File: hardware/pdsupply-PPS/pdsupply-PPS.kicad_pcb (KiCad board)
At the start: 4 copper layers, 44 x 36.5 mm, 74 parts, among them IC1 LTM8083EY#PBF, IC2 FPF2895UCX, J1 USB4505-03-0-A_REVA, J2 USB4505-03-0-A_REVA, J3 Screw_Terminal_01x02, U1 FUSB307BMPX, U2 ADUM3160, U3 ACS71240KEXBLT-050U5, U4 STM32L432KCUx

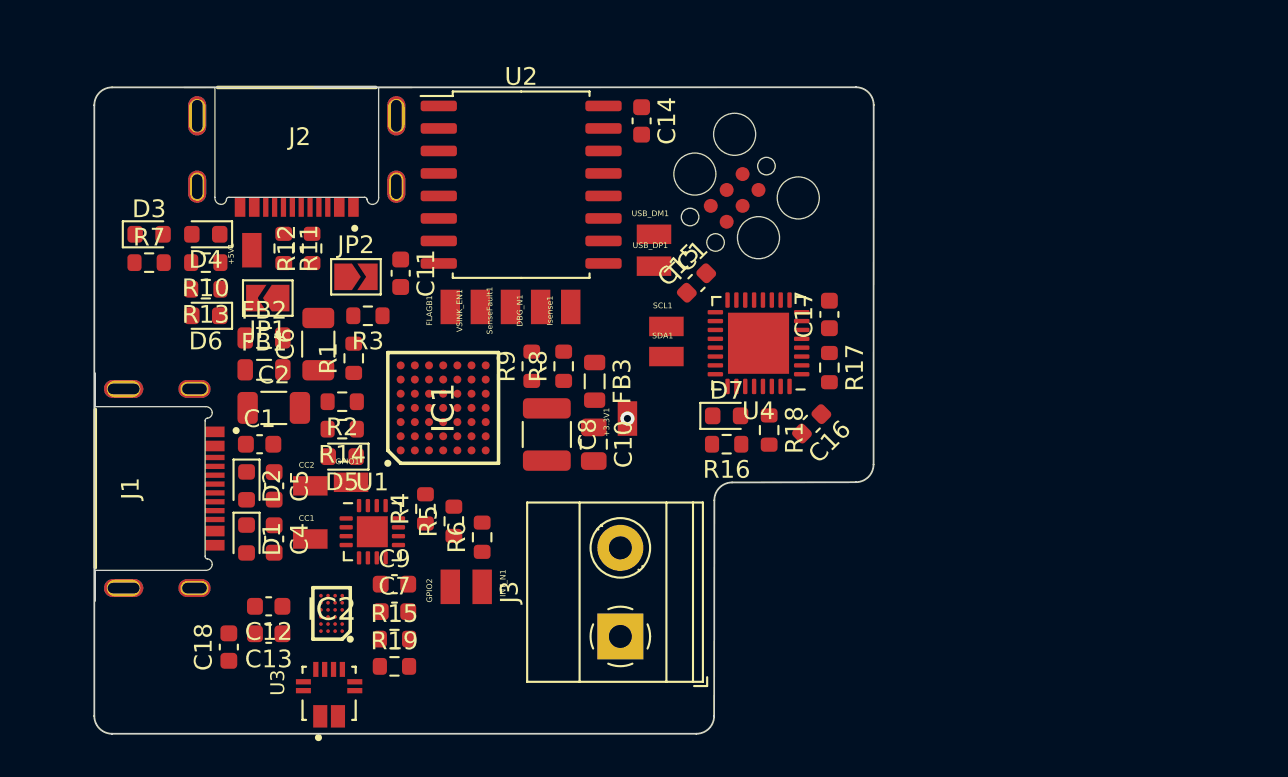
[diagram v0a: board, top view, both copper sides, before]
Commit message: added few routes
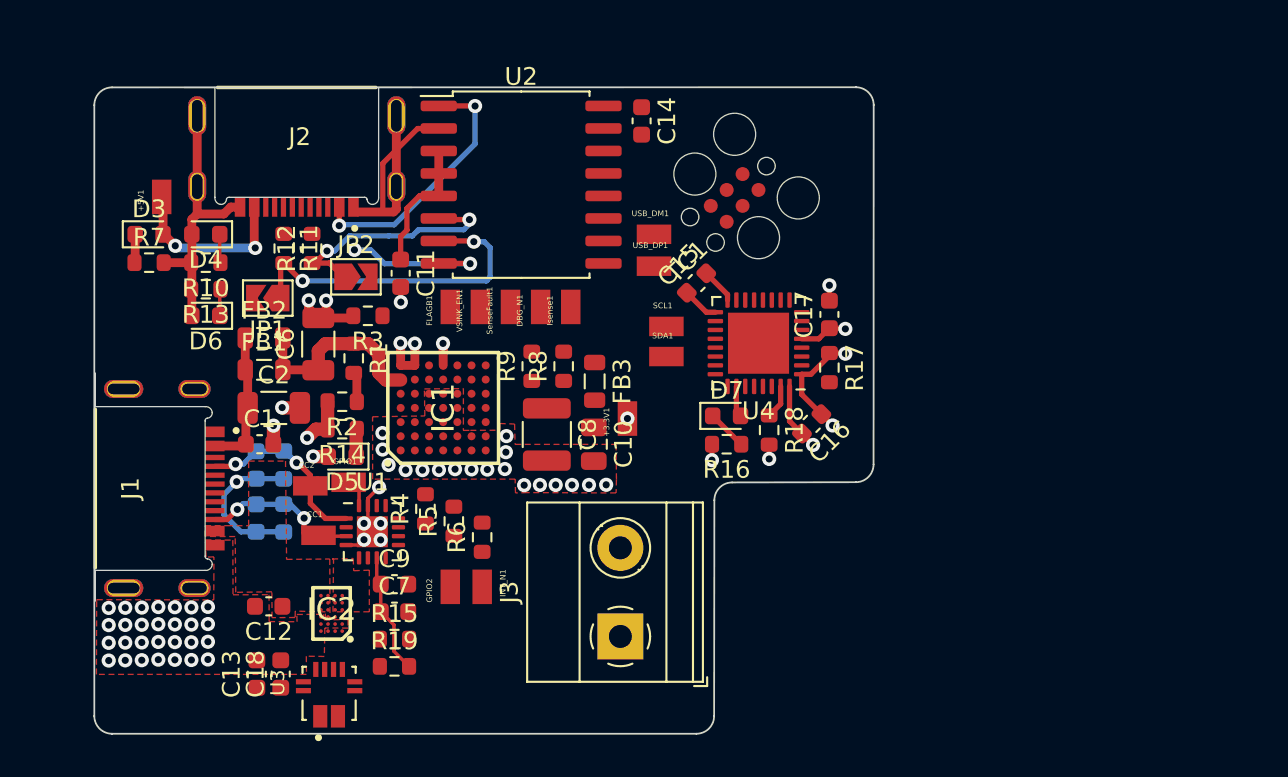
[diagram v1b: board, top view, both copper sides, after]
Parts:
- C4, C5, D1, D2: moved to B.Cu
- moved +5V1 5.91 mm to (113.8, 89.7)
- moved C18 3.30 mm to (120.5, 116.6)
- moved D1 2.41 mm to (120.7, 107.8)
- moved D2 2.41 mm to (120.7, 104.8)
- moved C13 2.37 mm to (119.2, 116.6), turned to 90 degrees
- moved C4 1.56 mm to (119.1, 107.8)
- moved C5 1.56 mm to (119.1, 104.8)
- moved CC1 0.51 mm to (122.7, 108.8)
- moved GPIO1 0.14 mm to (124.4, 105.8)
- turned R1 to -90 degrees
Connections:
- net Net-(C13-Pad1) renamed /Vbus_pre
- net Net-(J3-Pad1) renamed /VBus_Out
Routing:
- net GND1: track 0.00 -> 39.5 mm, vias 0 -> 3
- net GND: track 0.00 -> 35.1 mm, vias 0 -> 64
- net +5V: track 0.00 -> 24.9 mm, vias 0 -> 4
- net +3V3: track 0.00 -> 19.6 mm, vias 1 -> 5
- net Net-(JP1-Pad1): track 0.00 -> 18.9 mm, vias 0 -> 2
- net Net-(JP2-Pad1): track 0.00 -> 13.9 mm, vias 0 -> 2
- net Net-(C6-Pad1): track 0.00 -> 11.2 mm
- net /CC1: track 0.00 -> 10.7 mm, vias 0 -> 2
- net /CC2: track 0.00 -> 9.19 mm, vias 0 -> 2
- net VBUS: track 0.00 -> 8.20 mm
- net Net-(C11-Pad1): track 0.00 -> 7.66 mm
- net Net-(D7-Pad1): track 0.00 -> 2.28 mm
- net Net-(IC1-PadB6): track 0.00 -> 1.91 mm
- net Net-(R18-Pad1): track 0.00 -> 1.91 mm
- net Net-(D7-Pad2): track 0.00 -> 1.76 mm
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- added copper zone on F.Cu, net /Vbus_pre
- added copper zone on F.Cu, net GND
- added copper zone on F.Cu, net VBUS

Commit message: almost done with routing
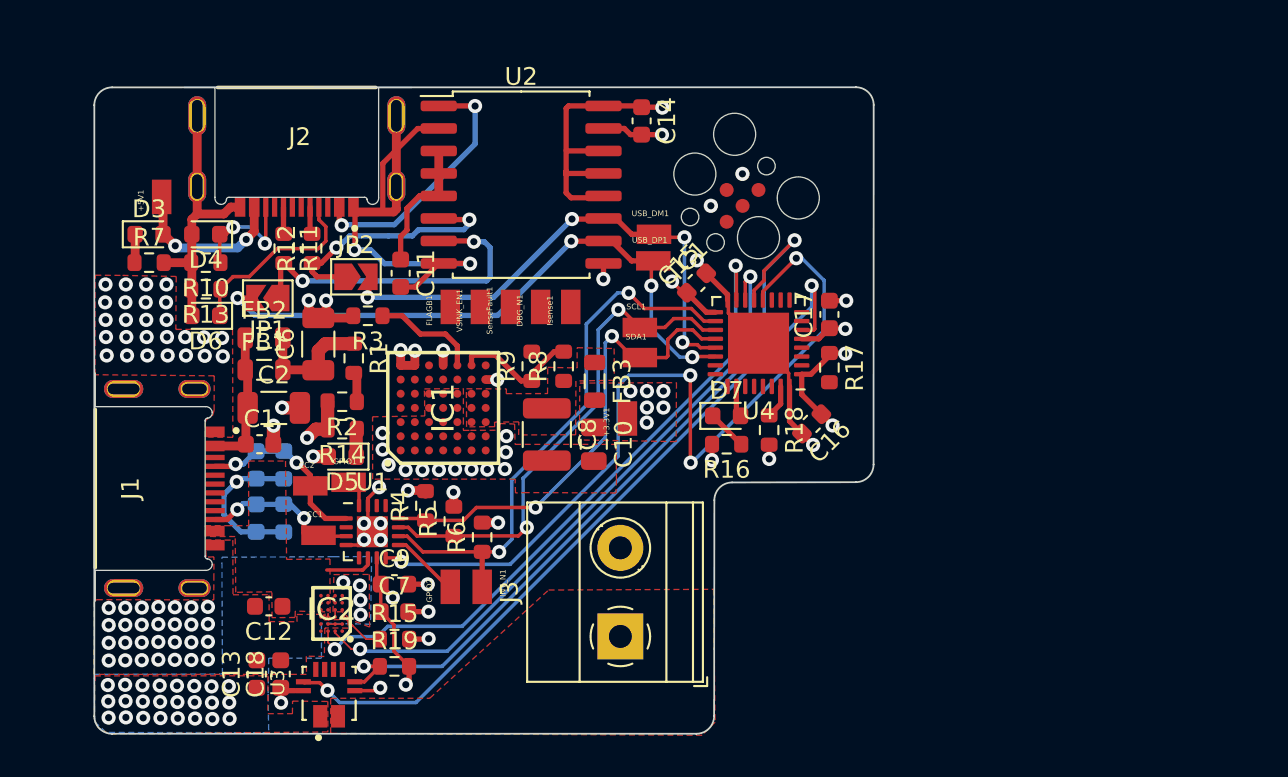
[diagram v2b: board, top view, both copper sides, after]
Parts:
- moved SCL1 1.50 mm to (140.8, 97.1)
- moved SDA1 1.50 mm to (140.8, 98.8)
- moved USB_DP1 0.30 mm to (141.6, 93.3)
- moved R4 0.17 mm to (128.7, 107.1)
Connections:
- net Net-(C8-Pad1) renamed /+3.3V_Pre
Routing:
- net /DBG_N: track 0.00 -> 47.7 mm, vias 0 -> 4
- net /SenseFault: track 0.00 -> 43.7 mm, vias 0 -> 2
- net /Isense: track 0.00 -> 42.8 mm, vias 0 -> 2
- net /FLAGB: track 0.00 -> 37.6 mm, vias 0 -> 2
- net /VSINK_EN: track 0.00 -> 36.5 mm, vias 0 -> 2
- net /USB_DP: track 0.00 -> 35.2 mm, vias 0 -> 4
- net /INT_N: track 0.00 -> 31.6 mm, vias 0 -> 2
- net /USB_DM: track 0.00 -> 29.8 mm, vias 0 -> 4
- net /SCL: track 0.00 -> 28.6 mm, vias 0 -> 2
- net /SDA: track 0.00 -> 27.0 mm, vias 0 -> 2
- net +3V3: track 19.6 -> 44.4 mm, vias 5 -> 19
- net GND: track 35.1 -> 53.4 mm, vias 64 -> 93
- net Net-(D6-Pad1): track 1.52 -> 10.7 mm
- net Net-(IC1-PadF7): track 0.00 -> 7.25 mm
- net Net-(IC1-PadE7): track 0.00 -> 6.03 mm
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- added copper zone on F.Cu, net +3V3
- added copper zone on F.Cu, net /+3.3V_Pre
- added copper zone on F.Cu, net /VBus_Out
- added copper zone on B.Cu, net /Vbus_pre

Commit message: almost done
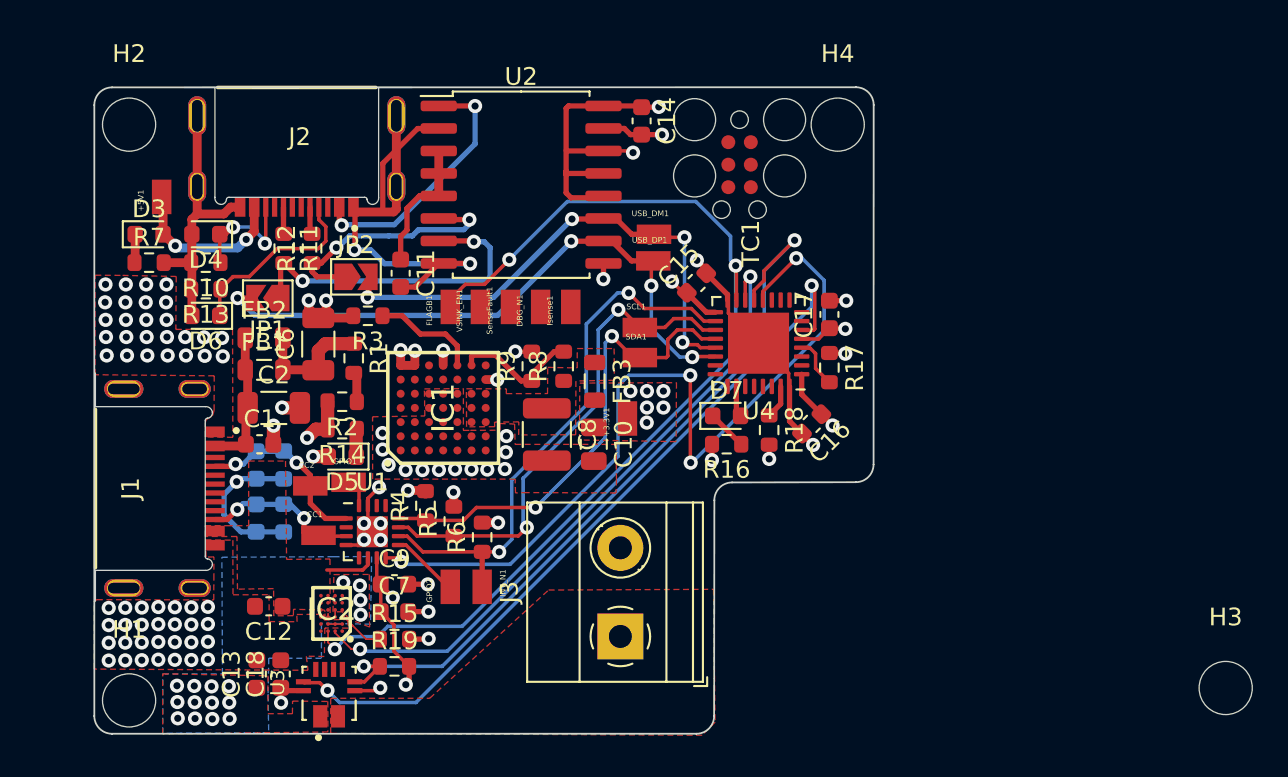
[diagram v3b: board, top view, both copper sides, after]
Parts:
- added H1: MountingHole_Pad, MountingHole:MountingHole_3mm, F.Cu at (112.0, 118.1)
- added H2: MountingHole_Pad, MountingHole:MountingHole_3mm, F.Cu at (112.0, 85.6)
- added H3: MountingHole_Pad, MountingHole:MountingHole_3mm, F.Cu at (173.9, 117.4)
- added H4: MountingHole_Pad, MountingHole:MountingHole_3mm, F.Cu at (152.0, 85.6)
- moved TC1 1.90 mm to (146.4, 87.9), turned to -90 degrees
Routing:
- net /FLAGB: track 37.6 -> 58.7 mm, vias 2 -> 3
- net Net-(R17-Pad2): track 0.00 -> 2.86 mm
- net GND: track 53.4 -> 54.4 mm
- net /Vbus_pre: vias 28 -> 16

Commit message: added holes
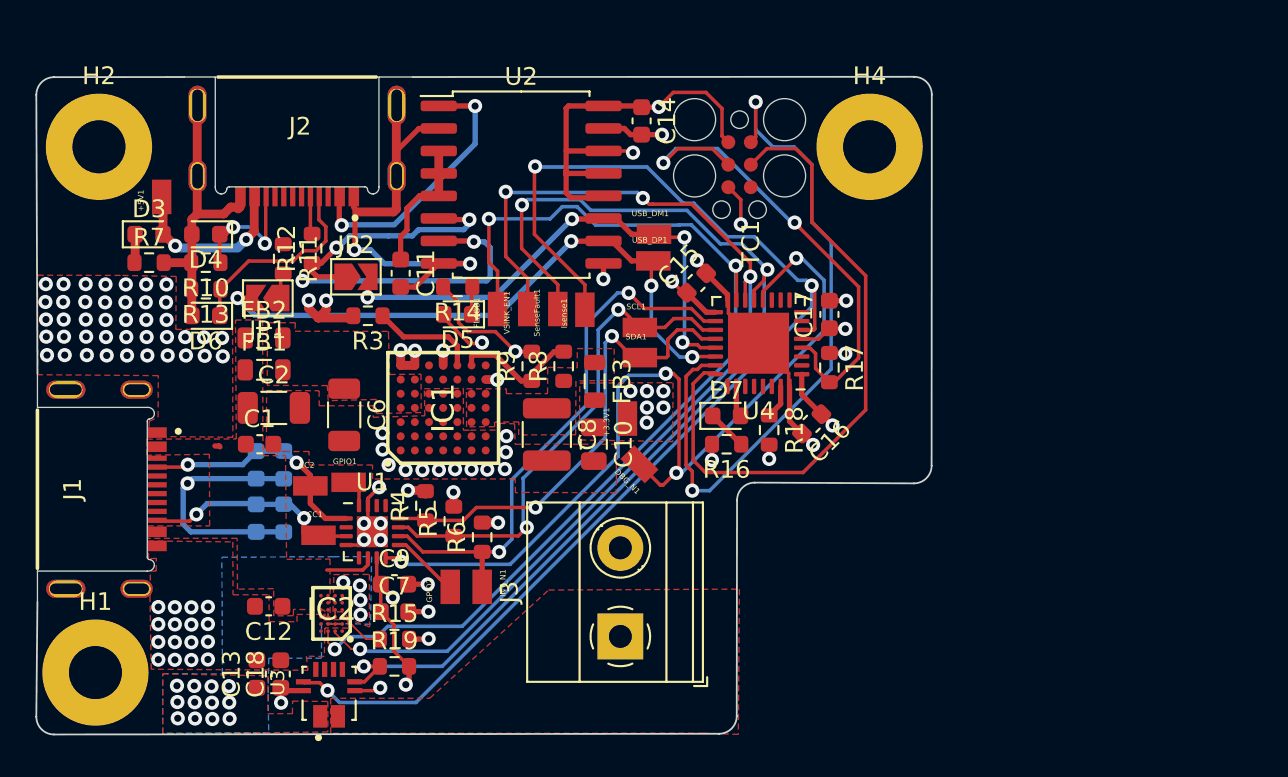
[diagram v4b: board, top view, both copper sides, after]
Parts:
- removed H3: MountingHole_Pad, MountingHole:MountingHole_3mm
- removed R1: 200k, Resistor_SMD:R_0603_1608Metric
- removed R2: 270k, Resistor_SMD:R_0603_1608Metric
- H1, H2, H4: footprint MountingHole:MountingHole_3mm -> MountingHole:MountingHole_3mm_Pad
- moved DBG_N1 10.5 mm to (140.8, 104.8), turned to 135 degrees
- moved D5 10.3 mm to (130.5, 96.3)
- moved R14 10.3 mm to (130.5, 94.8)
- moved C6 4.25 mm to (124.1, 102.0), turned to -90 degrees
- moved J1 3.27 mm to (108.4, 106.2)
- moved FLAGB1 2.67 mm to (132.8, 96.0)
- moved SenseFault1 2.67 mm to (136.2, 96.0)
- moved VSINK_EN1 2.67 mm to (134.5, 96.0)
- moved H1 2.46 mm to (110.1, 116.5)
- moved H4 2.19 mm to (153.8, 86.9)
- moved H2 2.11 mm to (110.3, 86.9)
- moved Isense1 0.82 mm to (137.7, 96.1)
- moved J2 0.59 mm to (121.5, 84.5)
- moved R11 0.59 mm to (120.7, 93.2)
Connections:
- C6 pad 1: Net-(C6-Pad1) -> /VBUS_Rdy
- FB1 pad 2: Net-(C6-Pad1) -> /VBUS_Rdy
- FB2 pad 2: Net-(C6-Pad1) -> /VBUS_Rdy
- IC1 pad A1: GND -> Net-(IC1-PadA1)
- IC1 pad A2: GND -> Net-(IC1-PadA1)
- IC1 pad A3: GND -> Net-(IC1-PadA1)
- IC1 pad A4: Net-(C6-Pad1) -> /VBUS_Rdy
- IC1 pad A5: Net-(C6-Pad1) -> /VBUS_Rdy
- IC1 pad A6: Net-(C6-Pad1) -> /VBUS_Rdy
- IC1 pad A7: GND -> Net-(IC1-PadA1)
- IC1 pad B1: GND -> Net-(IC1-PadA1)
- IC1 pad B2: GND -> Net-(IC1-PadA1)
- IC1 pad B3: GND -> Net-(IC1-PadA1)
- IC1 pad B4: Net-(C6-Pad1) -> /VBUS_Rdy
- IC1 pad B5: Net-(C6-Pad1) -> /VBUS_Rdy
- IC1 pad B6: Net-(IC1-PadB6) -> /VBUS_Rdy
- IC1 pad B7: GND -> Net-(IC1-PadA1)
- IC1 pad C1: GND -> Net-(IC1-PadA1)
- IC1 pad C2: GND -> Net-(IC1-PadA1)
- IC1 pad C3: GND -> Net-(IC1-PadA1)
- IC1 pad C4: GND -> Net-(IC1-PadA1)
- IC1 pad C5: GND -> Net-(IC1-PadA1)
- IC1 pad D1: GND -> Net-(IC1-PadA1)
- IC1 pad D2: GND -> Net-(IC1-PadA1)
- IC1 pad D3: GND -> Net-(IC1-PadA1)
- IC1 pad D4: GND -> Net-(IC1-PadA1)
- IC1 pad D5: GND -> Net-(IC1-PadA1)
- IC1 pad D7: GND -> Net-(IC1-PadA1)
- IC1 pad E1: GND -> Net-(IC1-PadA1)
- IC1 pad E2: GND -> Net-(IC1-PadA1)
- IC1 pad E3: GND -> Net-(IC1-PadA1)
- IC1 pad E4: GND -> Net-(IC1-PadA1)
- IC1 pad E5: GND -> Net-(IC1-PadA1)
- IC1 pad F1: GND -> Net-(IC1-PadA1)
- IC1 pad F2: GND -> Net-(IC1-PadA1)
- IC1 pad G1: GND -> Net-(IC1-PadA1)
- IC1 pad G2: GND -> Net-(IC1-PadA1)
- IC1 pad G6: GND -> Net-(IC1-PadA1)
- R3 pad 2: GND -> Net-(IC1-PadA1)
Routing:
- net Net-(TC1-Pad2): track 0.00 -> 39.1 mm, vias 0 -> 2
- net Net-(TC1-Pad4): track 0.00 -> 36.7 mm
- net /Isense: track 42.8 -> 70.4 mm, vias 2 -> 3
- net Net-(R17-Pad2): track 2.86 -> 28.1 mm, vias 0 -> 2
- net /VSINK_EN: track 36.5 -> 59.9 mm, vias 2 -> 4
- net /SenseFault: track 43.7 -> 61.5 mm, vias 2 -> 3
- net Net-(IC1-PadA1): track 0.00 -> 8.71 mm, vias 0 -> 6
- net +3V3: track 43.9 -> 52.4 mm
- net VBUS: track 11.2 -> 3.80 mm
- net Net-(C6-Pad1): track 7.07 -> 0.00 mm
- net /DBG_N: track 47.7 -> 51.6 mm
- net GND1: track 43.7 -> 39.9 mm
- net /CC2: track 9.19 -> 12.5 mm
- net /CC1: track 10.7 -> 14.0 mm
- net Net-(JP1-Pad1): track 18.9 -> 16.9 mm
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- added copper zone on F.Cu, net /VBUS_Rdy
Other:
- board size 44 x 36.5 mm -> 50.5 x 37.1 mm
